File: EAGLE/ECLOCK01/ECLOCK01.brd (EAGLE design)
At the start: 100 x 54 mm, 12 parts

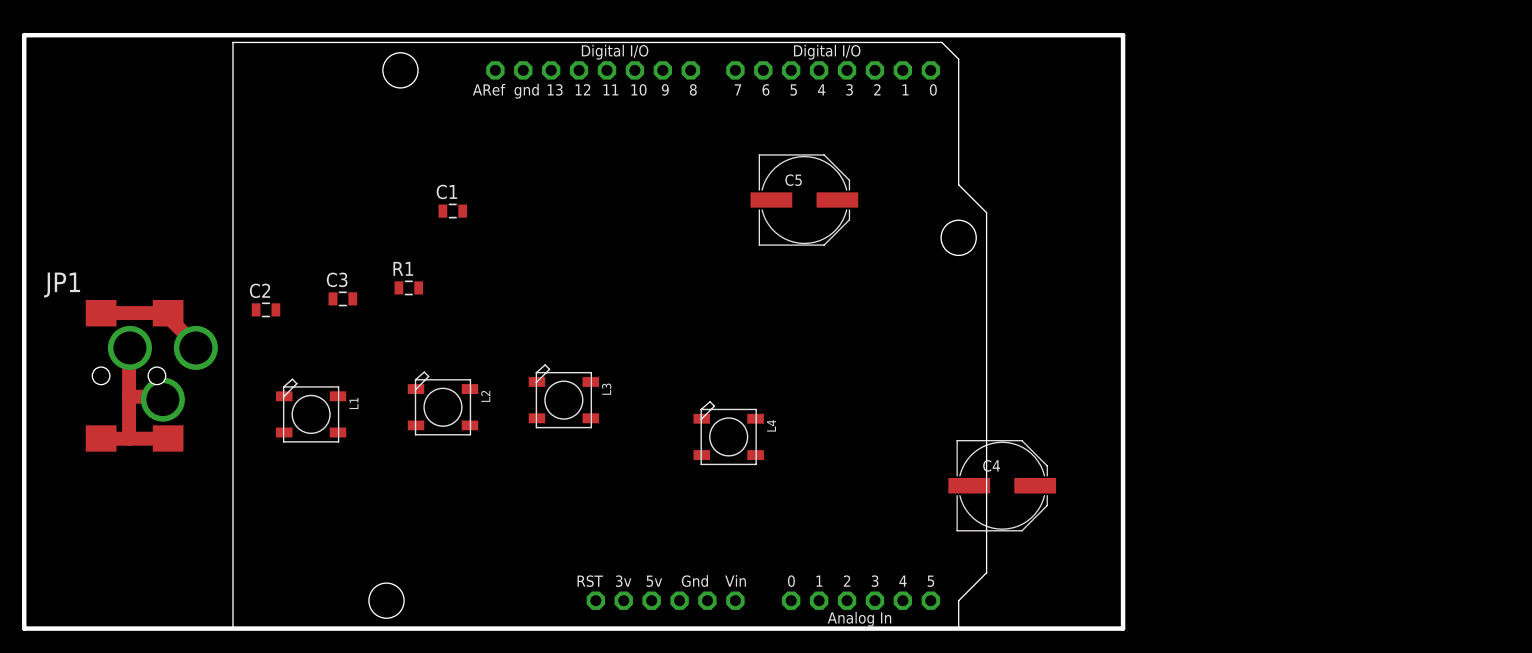
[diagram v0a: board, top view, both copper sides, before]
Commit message: FInal version of clock PCB before sending to board house
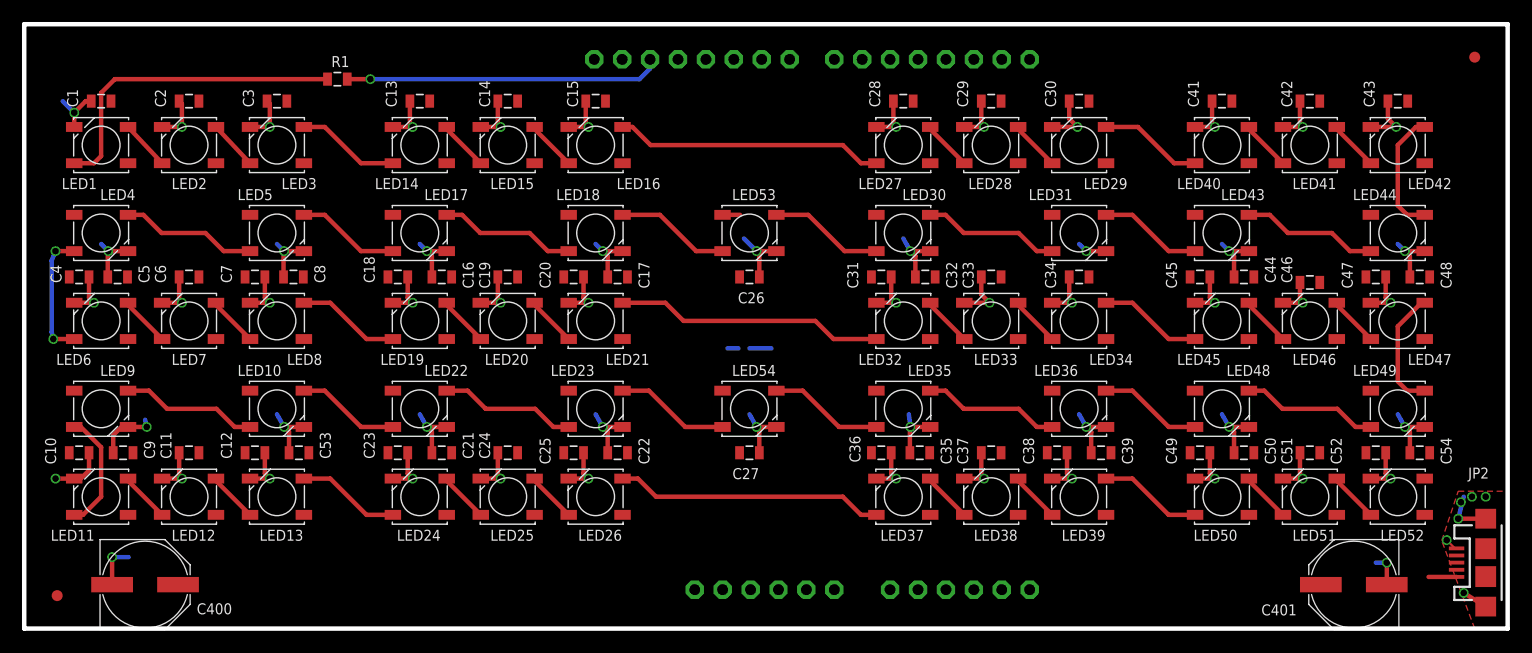
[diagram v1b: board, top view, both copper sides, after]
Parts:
- removed JP1: POWER_JACKCOMBO, SparkFun-Connectors:POWER_JACK_COMBO
- removed L1, L2, L3, L4: WS2812B, adafruit:WS2812B
- added C10, C11, C12, C13, C14, C15, C16, C17, C18, C19, C20, C21, C22, C23, C24, C25, C26, C27, C28, C29, C30, C31, C32, C33, C34, C35, C36, C37, C38, C39, C41, C42, C43, C44, C45, C46, C47, C48, C49, C50, C51, C52, C53, C54, C6, C7, C8, C9: 0.1, TinWhiskers:0805
- added C400, C401: 470, adafruit:PANASONIC_E
- added FID1, FID2: FIDUCIAL, TinWhiskers:FIDUCIAL
- added JP2: USB-MICROB, SparkFun-Connectors:USB-MICROB
- added LED1, LED10, LED11, LED12, LED13, LED14, LED15, LED16, LED17, LED18, LED19, LED2, LED20, LED21, LED22, LED23, LED24, LED25, LED26, LED27, LED28, LED29, LED3, LED30, LED31, LED32, LED33, LED34, LED35, LED36, LED37, LED38, LED39, LED4, LED40, LED41, LED42, LED43, LED44, LED45, LED46, LED47, LED48, LED49, LED5, LED50, LED51, LED52, LED53, LED54, LED6, LED7, LED8, LED9: WS2812B, GinWhiskers - temp stuff:WS2812B
- C1, C2, C3: value CAPACITOR0805 -> 0.1
- C4, C5: value 470 -> 0.1; device adafruit:PANASONIC_E -> TinWhiskers:0805
- U$1: device adafruit:ARDUINO -> GinWhiskers - temp stuff:ARDUINO-UNO
- moved C4 86.1 mm to (5.00, 32.0)
- moved C5 62.9 mm to (8.50, 32.0), turned to 180 degrees
- moved C1 33.5 mm to (7.00, 48.0), turned to 180 degrees
- moved C2 20.2 mm to (15.0, 48.0), turned to 180 degrees
- moved R1 20.1 mm to (28.5, 50.0), turned to 180 degrees
- moved C3 19.0 mm to (23.0, 48.0), turned to 180 degrees
- moved U$1 9.06 mm to (28.0, 1.00)
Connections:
- removed net N$6: L3.2-DOUT, L4.4-DIN
- new net N$10: LED15.2-DOUT, LED16.4-DIN
- new net N$12: LED18.4-DIN, LED53.2-DOUT
- new net N$13: LED19.2-DOUT, LED20.4-DIN
- new net N$14: LED17.4-DIN, LED18.2-DOUT
- new net N$15: LED19.4-DIN, LED8.2-DOUT
- new net N$16: LED47.2-DOUT, LED49.4-DIN
- new net N$17: LED39.2-DOUT, LED50.4-DIN
- new net N$18: LED24.2-DOUT, LED25.4-DIN
- new net N$19: LED25.2-DOUT, LED26.4-DIN
- new net N$2: LED11.2-DOUT, LED12.4-DIN
- new net N$20: LED13.2-DOUT, LED24.4-DIN
- new net N$21: LED27.2-DOUT, LED28.4-DIN
- new net N$22: LED28.2-DOUT, LED29.4-DIN
- new net N$25: LED40.2-DOUT, LED41.4-DIN
- new net N$26: LED20.2-DOUT, LED21.4-DIN
- new net N$27: LED11.4-DIN, LED9.2-DOUT
- new net N$28: LED17.2-DOUT, LED5.4-DIN
- new net N$29: LED4.4-DIN, LED5.2-DOUT
- new net N$30: LED6.2-DOUT, LED7.4-DIN
- new net N$31: LED7.2-DOUT, LED8.4-DIN
- new net N$32: LED21.2-DOUT, LED32.4-DIN
- new net N$33: LED48.4-DIN, LED49.2-DOUT
- new net N$34: LED36.4-DIN, LED48.2-DOUT
- new net N$36: LED37.2-DOUT, LED38.4-DIN
- new net N$37: LED38.2-DOUT, LED39.4-DIN
- new net N$39: LED30.2-DOUT, LED53.4-DIN
- new net N$40: LED34.2-DOUT, LED45.4-DIN
- new net N$41: LED32.2-DOUT, LED33.4-DIN
- new net N$42: LED33.2-DOUT, LED34.4-DIN
- new net N$44: LED31.4-DIN, LED43.2-DOUT
- new net N$45: LED4.2-DOUT, LED6.4-DIN
- new net N$46: LED46.2-DOUT, LED47.4-DIN
- new net N$47: LED45.2-DOUT, LED46.4-DIN
- new net N$48: LED42.2-DOUT, LED44.4-DIN
- new net N$49: LED43.4-DIN, LED44.2-DOUT
- new net N$50: LED30.4-DIN, LED31.2-DOUT
- new net N$51: LED41.2-DOUT, LED42.4-DIN
- new net N$52: LED35.4-DIN, LED36.2-DOUT
- new net N$53: LED35.2-DOUT, LED54.4-DIN
- new net N$54: LED50.2-DOUT, LED51.4-DIN
- new net N$55: LED51.2-DOUT, LED52.4-DIN
- new net N$56: LED23.4-DIN, LED54.2-DOUT
- new net N$58: LED22.4-DIN, LED23.2-DOUT
- new net N$59: LED14.4-DIN, LED3.2-DOUT
- new net N$60: LED10.4-DIN, LED22.2-DOUT
- new net N$61: LED10.2-DOUT, LED9.4-DIN
- new net N$62: LED29.2-DOUT, LED40.4-DIN
- new net N$7: LED12.2-DOUT, LED13.4-DIN
- new net N$8: LED26.2-DOUT, LED37.4-DIN
- new net N$9: LED14.2-DOUT, LED15.4-DIN
- new net VDD: C1.1, C10.1, C11.1, C12.1, C13.1, C14.1, C15.1, C16.1, C17.1, C18.1, C19.1, C2.1, C20.1, C21.1, C22.1, C23.1, C24.1, C25.1, C26.1, C27.1, C28.1, C29.1, C3.1, C30.1, C31.1, C32.1, C33.1, C34.1, C35.1, C36.1, C37.1, C38.1, C39.1, C4.1, C400.+, C401.+, C41.1, C42.1, C43.1, C44.1, C45.1, C46.1, C47.1, C48.1, C49.1, C5.1, C50.1, C51.1, C52.1, C53.1, C54.1, C6.1, C7.1, C8.1, C9.1, JP2.VBUS, LED1.1-VDD, LED10.1-VDD, LED11.1-VDD, LED12.1-VDD, LED13.1-VDD, LED14.1-VDD, LED15.1-VDD, LED16.1-VDD, LED17.1-VDD, LED18.1-VDD, LED19.1-VDD, LED2.1-VDD, LED20.1-VDD, LED21.1-VDD, LED22.1-VDD, LED23.1-VDD, LED24.1-VDD, LED25.1-VDD, LED26.1-VDD, LED27.1-VDD, LED28.1-VDD, LED29.1-VDD, LED3.1-VDD, LED30.1-VDD, LED31.1-VDD, LED32.1-VDD, LED33.1-VDD, LED34.1-VDD, LED35.1-VDD, LED36.1-VDD, LED37.1-VDD, LED38.1-VDD, LED39.1-VDD, LED4.1-VDD, LED40.1-VDD, LED41.1-VDD, LED42.1-VDD, LED43.1-VDD, LED44.1-VDD, LED45.1-VDD, LED46.1-VDD, LED47.1-VDD, LED48.1-VDD, LED49.1-VDD, LED5.1-VDD, LED50.1-VDD, LED51.1-VDD, LED52.1-VDD, LED53.1-VDD, LED54.1-VDD, LED6.1-VDD, LED7.1-VDD, LED8.1-VDD, LED9.1-VDD
- net GND: now also C1.2, C10.2, C11.2, C12.2, C13.2, C14.2, C15.2, C16.2, C17.2, C18.2, C19.2, C2.2, C20.2, C21.2, C22.2, C23.2, C24.2, C25.2, C26.2, C27.2, C28.2, C29.2, C3.2, C30.2, C31.2, C32.2, C33.2, C34.2, C35.2, C36.2, C37.2, C38.2, C39.2, C4.2, C400.-, C401.-, C41.2, C42.2, C43.2, C44.2, C45.2, C46.2, C47.2, C48.2, C49.2, C5.2, C50.2, C51.2, C52.2, C53.2, C54.2, C6.2, C7.2, C8.2, C9.2, JP2.GND, JP2.MT1, JP2.MT2, LED1.3-GND, LED10.3-GND, LED11.3-GND, LED12.3-GND, LED13.3-GND, LED14.3-GND, LED15.3-GND, LED16.3-GND, LED17.3-GND, LED18.3-GND, LED19.3-GND, LED2.3-GND, LED20.3-GND, LED21.3-GND, LED22.3-GND, LED23.3-GND, LED24.3-GND, LED25.3-GND, LED26.3-GND, LED27.3-GND, LED28.3-GND, LED29.3-GND, LED3.3-GND, LED30.3-GND, LED31.3-GND, LED32.3-GND, LED33.3-GND, LED34.3-GND, LED35.3-GND, LED36.3-GND, LED37.3-GND, LED38.3-GND, LED39.3-GND, LED4.3-GND, LED40.3-GND, LED41.3-GND, LED42.3-GND, LED43.3-GND, LED44.3-GND, LED45.3-GND, LED46.3-GND, LED47.3-GND, LED48.3-GND, LED49.3-GND, LED5.3-GND, LED50.3-GND, LED51.3-GND, LED52.3-GND, LED53.3-GND, LED54.3-GND, LED6.3-GND, LED7.3-GND, LED8.3-GND, LED9.3-GND; no longer C4.-, C5.-, JP1.GND, JP1.GND@1, L1.3-GND, L2.3-GND, L3.3-GND, L4.3-GND
- net LED_IN: now also U$1.D13; no longer U$1.D0
- net N$1: now also LED1.4-DIN; no longer L1.4-DIN
- net N$3: now also LED1.2-DOUT, LED2.4-DIN; no longer L1.2-DOUT, L2.4-DIN
- net N$4: now also LED2.2-DOUT, LED3.4-DIN; no longer L2.2-DOUT, L3.4-DIN
- net N$5: now also LED16.2-DOUT, LED27.4-DIN; no longer C4.+, C5.+, JP1.POWER, L1.1-VDD, L2.1-VDD, L3.1-VDD, L4.1-VDD
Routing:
- net GND: track 0.00 -> 271.3 mm, vias 0 -> 62
- net N$1: track 0.00 -> 29.6 mm
- net LED_IN: track 0.00 -> 28.8 mm, vias 0 -> 1
- net N$8: track 0.00 -> 24.5 mm
- net N$5: track 0.00 -> 24.5 mm
- net N$32: track 0.00 -> 24.5 mm
- net N$61: track 0.00 -> 12.5 mm
- net N$29: track 0.00 -> 12.5 mm
- net N$58: track 0.00 -> 12.5 mm
- net N$14: track 0.00 -> 12.5 mm
- net N$52: track 0.00 -> 12.5 mm
- net N$50: track 0.00 -> 12.5 mm
- net N$49: track 0.00 -> 12.5 mm
- net N$33: track 0.00 -> 12.5 mm
- net N$45: track 0.00 -> 11.7 mm, vias 0 -> 2
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- added copper zone on layer 1, net GND
- added copper zone on layer 16, net GND
- added copper zone on layer 1, net VDD
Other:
- board size 100 x 54 mm -> 135 x 55 mm
